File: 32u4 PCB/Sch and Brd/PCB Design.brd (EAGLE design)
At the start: 95.8 x 64.6 mm, 57 parts, among them J1 AVR_SPI_PROG_3X2PTH, J2 AMP FCI 10103594-0001LF, Q1 16MHz, U1 ATMEGA32U4-AU

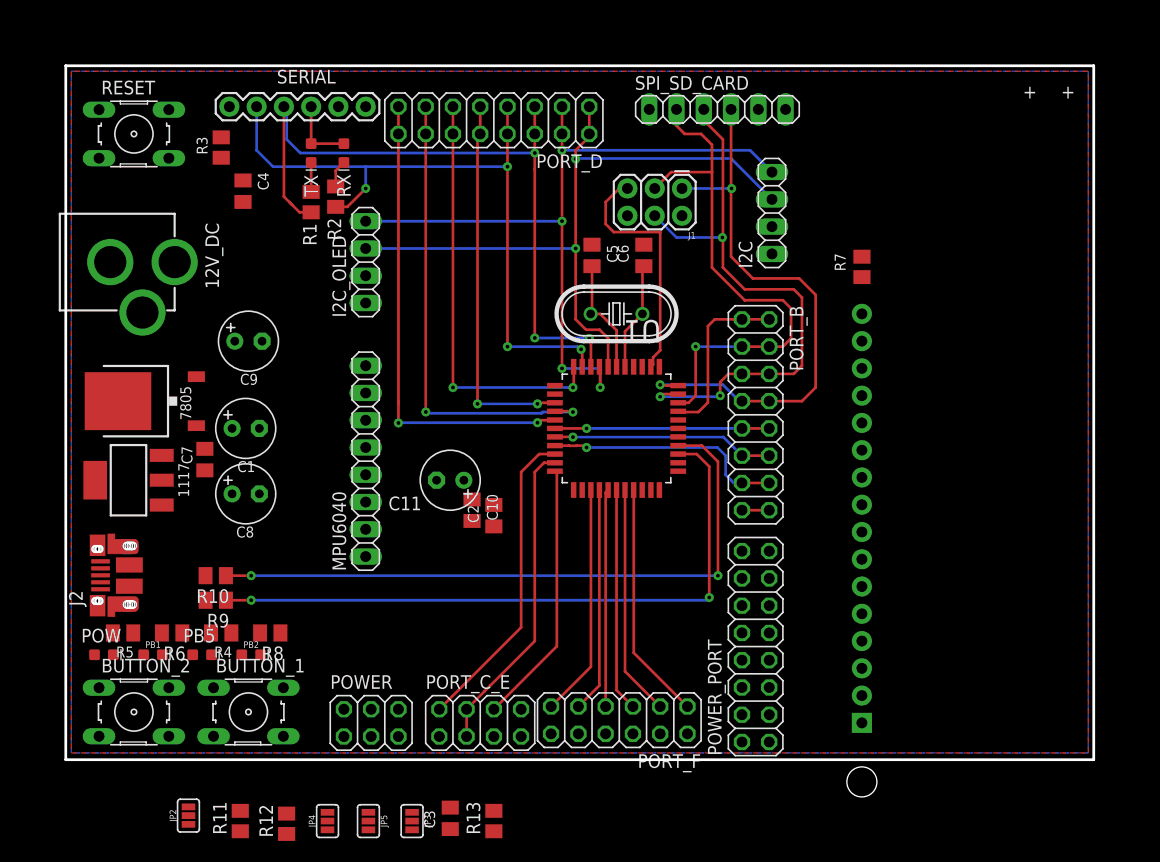
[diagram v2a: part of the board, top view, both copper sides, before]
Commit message: Rough layout ready
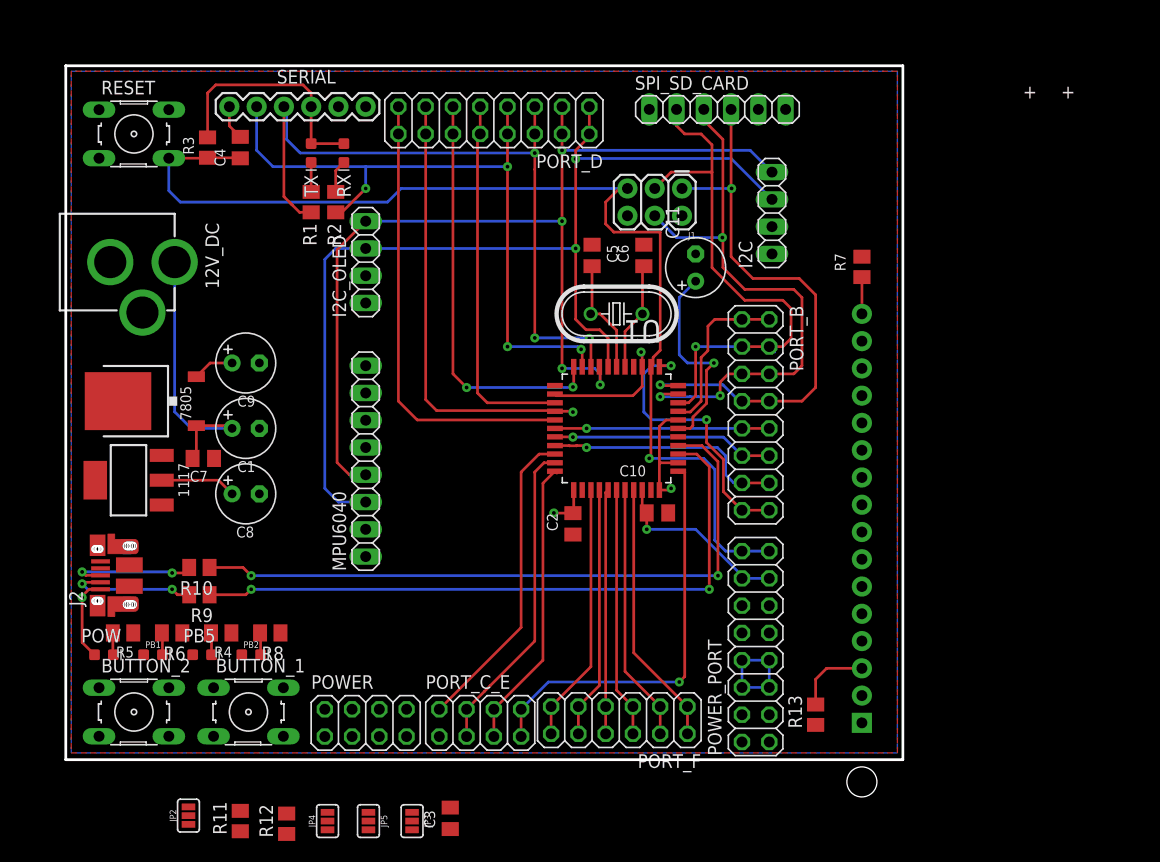
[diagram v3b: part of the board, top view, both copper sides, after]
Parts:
- POWER: device pinhead:2X03 -> pinhead:2X04
- moved R13 31.6 mm to (77.2, 9.91)
- moved C11 30.3 mm to (66.0, 51.6), turned to 90 degrees
- moved C10 17.3 mm to (62.5, 28.7), turned to 0 degrees
- moved C2 7.41 mm to (54.6, 27.7)
- moved C4 4.07 mm to (23.6, 62.7), turned to 90 degrees
- moved C9 2.05 mm to (24.1, 42.7)
- moved R10 1.70 mm to (19.8, 23.6)
- moved R9 1.61 mm to (19.8, 21.1)
- moved R3 1.27 mm to (20.6, 62.7)
- moved POWER 0.51 mm to (35.3, 9.14)
- moved R2 0.51 mm to (32.5, 57.7)
- moved C7 0.18 mm to (20.2, 33.8), turned to 0 degrees
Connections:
- net +5V: now also POWER.3, POWER.4
- net AREF: no longer POWER.3, POWER.4
- net GND: now also POWER.7, POWER.8
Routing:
- net RESET: track 22.9 -> 103.5 mm, vias 0 -> 1
- net +5V: track 6.49 -> 60.6 mm, vias 0 -> 4
- net PE6: track 0.00 -> 38.7 mm, vias 0 -> 1
- net PD0/SCL: track 66.2 -> 96.1 mm
- net +12V: track 0.00 -> 26.6 mm
- net PD1/SDA: track 70.2 -> 96.3 mm
- net PB7: track 2.54 -> 26.0 mm, vias 0 -> 2
- net N$16: track 0.00 -> 19.2 mm, vias 0 -> 1
- net AREF: track 0.00 -> 17.3 mm, vias 0 -> 1
- net D-: track 0.00 -> 12.2 mm, vias 0 -> 2
- net D+: track 0.00 -> 12.1 mm, vias 0 -> 2
- net 3V3: track 0.00 -> 10.2 mm
- net N$6: track 0.00 -> 7.09 mm
- net 3.3V: track 0.00 -> 7.08 mm
- net N$14: track 0.00 -> 3.43 mm
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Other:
- board size 95.8 x 64.6 mm -> 78 x 64.6 mm

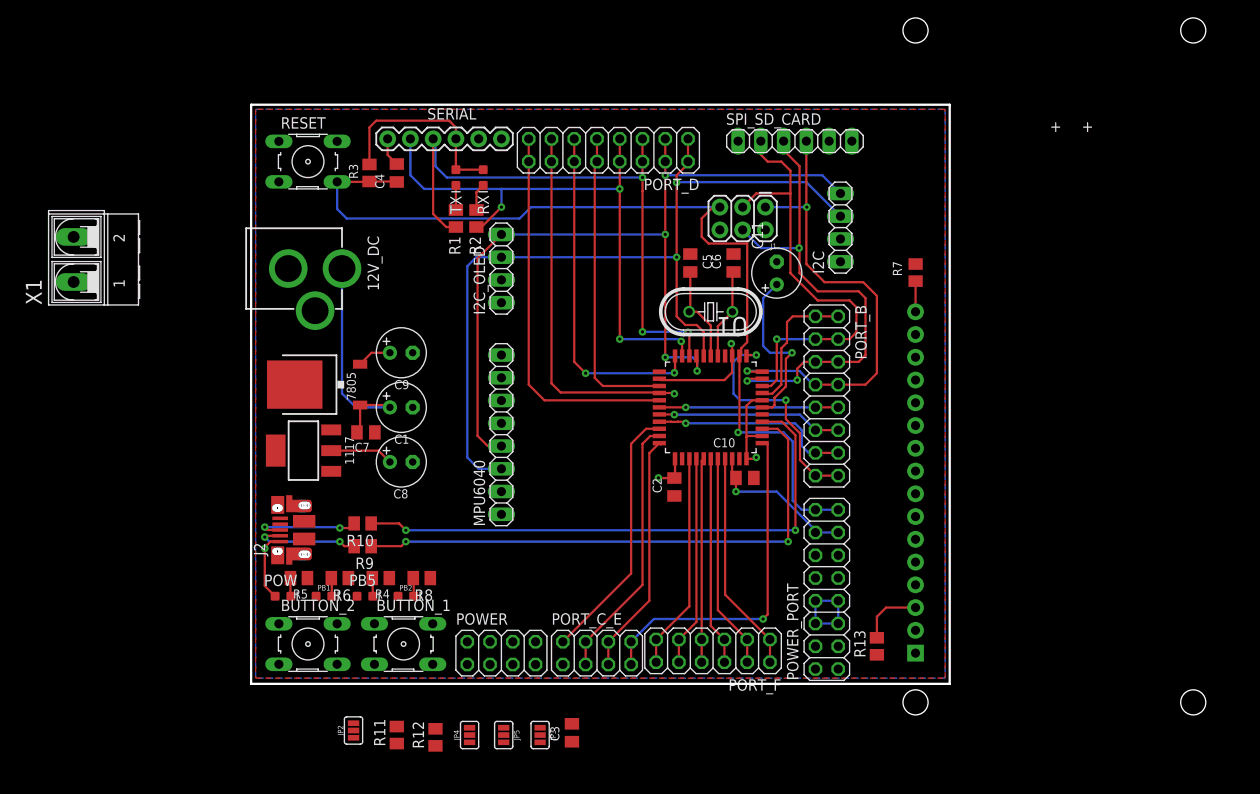
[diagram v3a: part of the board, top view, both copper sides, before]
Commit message: Routing almost done
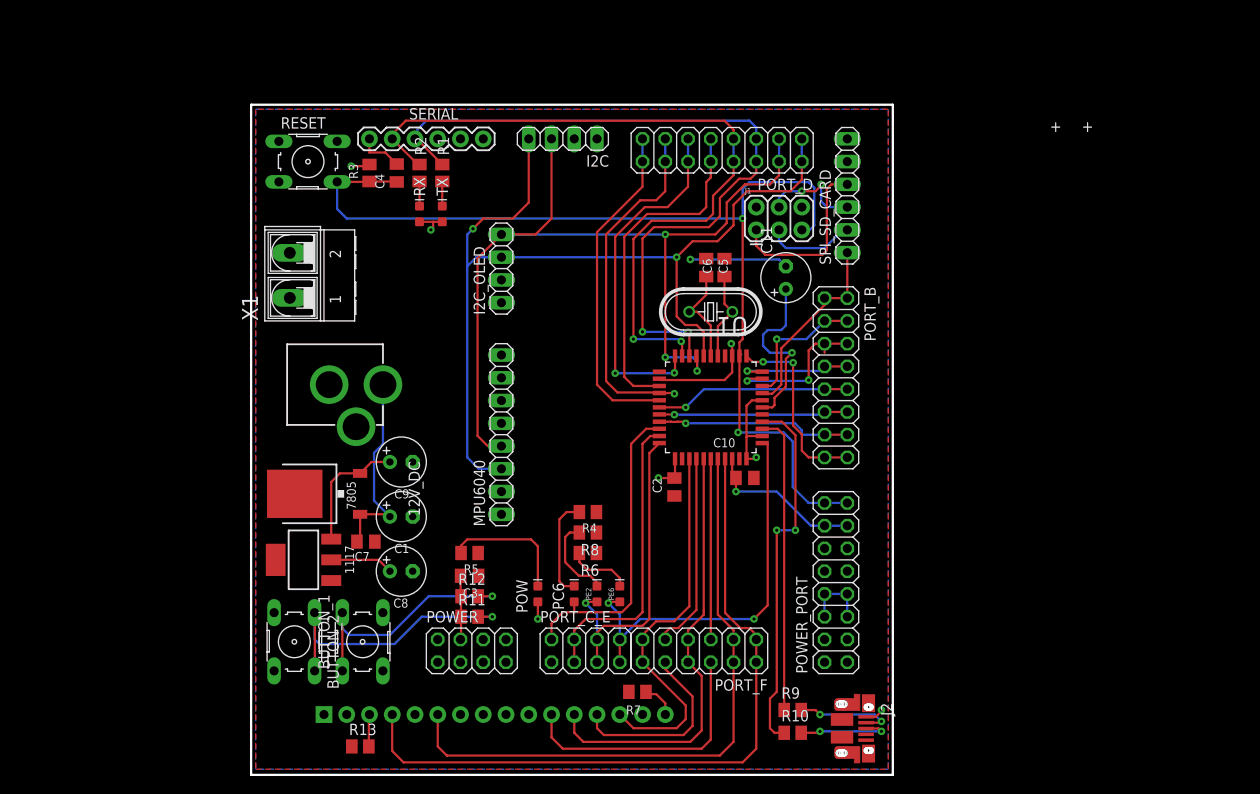
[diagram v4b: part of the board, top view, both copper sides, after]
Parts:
- removed JP2, JP3, JP4, JP5: JUMPER-SMT_3_1-NC_PASTE_SILK, SparkFun-Jumpers:SMT-JUMPER_3_1-NC_PASTE_SILK
- removed PB1, PB2, PB5: Yellow, SparkFun-LED:LED-0603
- added PC6, PE2, PE6: Yellow, SparkFun-LED:LED-0603
- LCD1: value LCD-16X2NOSILK -> LCD-16X2NOHOLES; device SparkFun-Displays:LCD-16X2_NOSILK -> SparkFun-Displays:LCD-16X2_NOHOLESNOSILK
- R4, R5, R6, R8: value 1K -> 330
- moved LCD1 73.5 mm to (47.5, -13.2), turned to 0 degrees
- moved J2 66.5 mm to (74.7, 0.76), turned to 270 degrees
- moved R13 58.7 mm to (19.6, -1.27), turned to 0 degrees
- moved R7 56.2 mm to (50.5, 4.83), turned to 0 degrees
- moved R10 53.4 mm to (67.8, 0.25), turned to 0 degrees
- moved R9 51.4 mm to (67.8, 2.79), turned to 0 degrees
- moved I2C 32.5 mm to (42.2, 66.5), turned to 180 degrees
- moved POW 28.4 mm to (39.4, 15.7), turned to 90 degrees
- moved R6 27.8 mm to (45.0, 20.3)
- moved R4 24.3 mm to (45.0, 24.9)
- moved X1 24.2 mm to (11.7, 51.3)
- moved C3 20.9 mm to (31.8, 17.8), turned to 0 degrees
- moved R5 19.3 mm to (31.8, 20.3)
- moved R8 19.2 mm to (45.0, 22.6)
- moved R12 16.2 mm to (31.8, 15.5), turned to 0 degrees
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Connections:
- removed net CS: SPI_SD_CARD.1
- removed net D4: LCD1.11
- removed net D5: LCD1.12
- removed net D6: LCD1.13
- removed net D7: LCD1.14
- removed net E: LCD1.6
- removed net N$10: PB1.A
- removed net N$11: PB2.A
- removed net N$12: PB5.A
- removed net N$17: JP2.2, R11.1
- removed net N$18: BUTTON_1.3, BUTTON_1.4, JP3.2
- removed net N$19: BUTTON_2.3, BUTTON_2.4, JP5.2
- removed net N$20: JP4.2, R12.1
- removed net PB0: PORT_B.1, PORT_B.2, U1.8
- removed net RS: LCD1.4
- new net PB0/SS: PORT_B.1, PORT_B.2, SPI_SD_CARD.1, U1.8
- net +5V: now also R11.1, R12.1; no longer JP2.1, JP3.3, JP4.1, JP5.3
- net GND: now also BUTTON_1.3, BUTTON_1.4, BUTTON_2.3, BUTTON_2.4; no longer JP2.3, JP3.1, JP4.3, JP5.1
- net N$1: now also PC6.C; no longer PB5.C
- net N$3: now also PE6.C; no longer PB1.C
- net N$7: now also PE2.C; no longer PB2.C
- net PC6: now also PC6.A
- net PD0/SCL: now also I2C.4; no longer I2C.3
- net PD1/SDA: now also I2C.3; no longer I2C.4
- net PE2: now also PE2.A
- net PE6: now also PE6.A
- net PF0: now also LCD1.4
- net PF1: now also LCD1.6
- net PF4/TCK: now also LCD1.11
- net PF5/TMS: now also LCD1.12
- net PF6/TDO: now also LCD1.13
- net PF7/TDI: now also LCD1.14
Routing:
- net PIN: track 0.00 -> 61.1 mm, vias 0 -> 2
- net PF0: track 24.8 -> 80.3 mm
- net PF1: track 24.1 -> 70.0 mm
- net N$13: track 61.6 -> 33.4 mm, vias 2 -> 0
- net PF4/TCK: track 23.3 -> 50.1 mm
- net PF5/TMS: track 22.8 -> 48.9 mm
- net PB2/MOSI: track 54.6 -> 29.3 mm, vias 3 -> 4
- net PB1/SCK: track 51.2 -> 26.6 mm
- net PB0/SS: track 0.00 -> 21.9 mm
- net N$15: track 62.6 -> 41.2 mm
- net PB3/MISO: track 53.7 -> 32.7 mm, vias 2 -> 1
- net PF6/TDO: track 23.5 -> 43.5 mm
- net PF7/TDI: track 24.2 -> 42.8 mm
- net PD3/TXD1: track 64.8 -> 82.6 mm, vias 4 -> 2
- net PB0: track 16.6 -> 0.00 mm
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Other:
- board size 78 x 64.6 mm -> 71.6 x 74.8 mm
